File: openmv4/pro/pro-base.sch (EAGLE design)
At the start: 172 parts, among them J2 SAMTEC_FTSH-105-01-F-DVSAMTEC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, J6 RSP-122811-01, M1 9774030243R, M2 9774030243R, Q1 BSS138, Q2 AO3401, U1 W25Q256JVEIQ_TR, U10 STM32H743IIK6, U11 TEXAS_INSTRUMENTS_BQ24072TRGT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, U12 MICROCHIP_ATECC608A-SSHDA-BMI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, U14 IS42S32800, U2 EMIF06-MSD02N16, U3 ME6211C18M5G, U4 PAM2305AABADJ, U5 LSM6DS3TR-C, U6 MICROCHIP_USB3320C-EZK-TRMICR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, U7 LBEE5KL1DX-TEMP, U9 VL53L5CX, X2 USD-1040310811, X3 DF12-36-DS, X4 S2B-PH-K-S(LF)(SN), Y0 SITIME_SIT1533AI-H4-DCC-32.76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, Y1 DSC1001BI1-024.0000

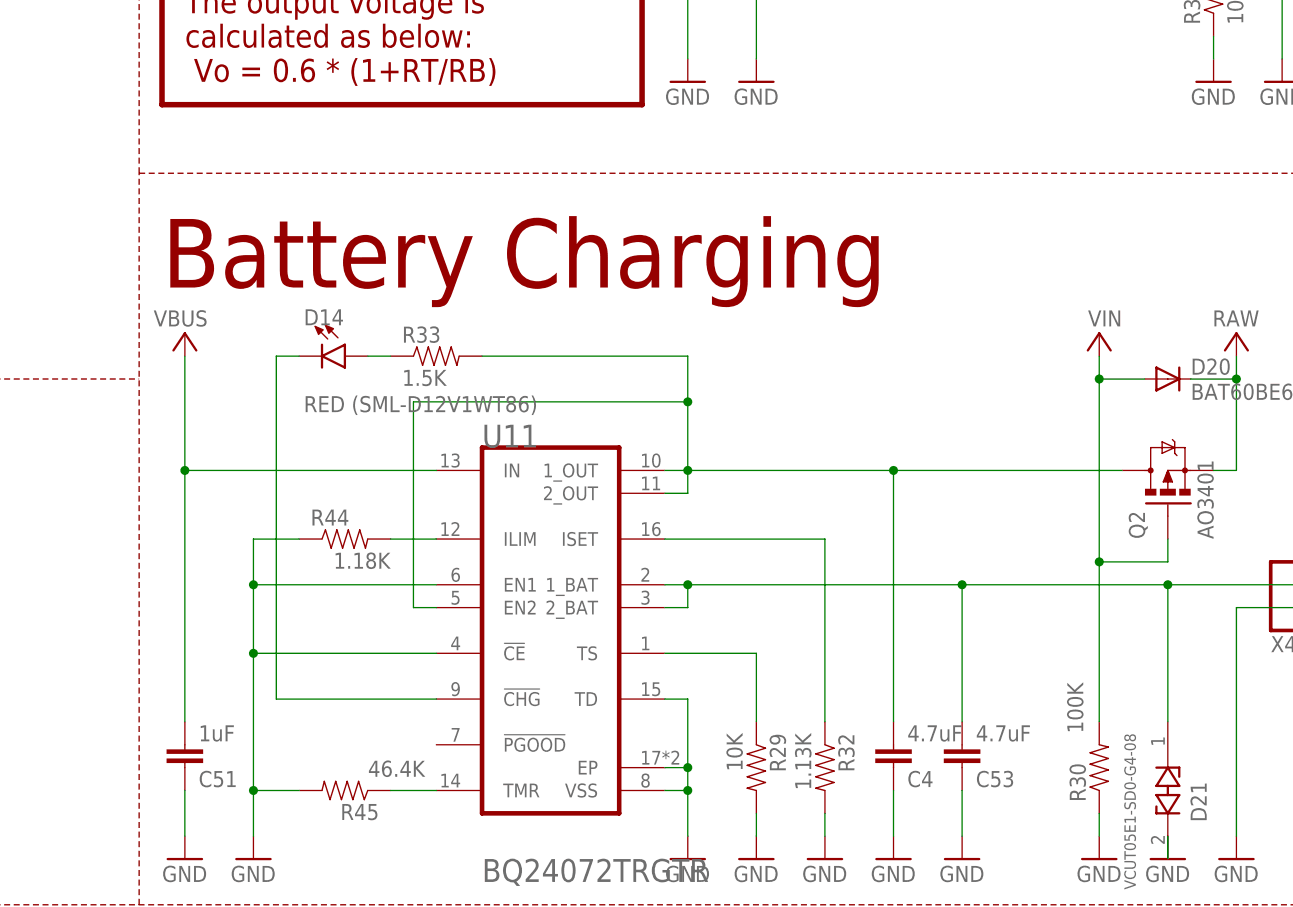
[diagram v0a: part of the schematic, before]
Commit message: Update pro schematics
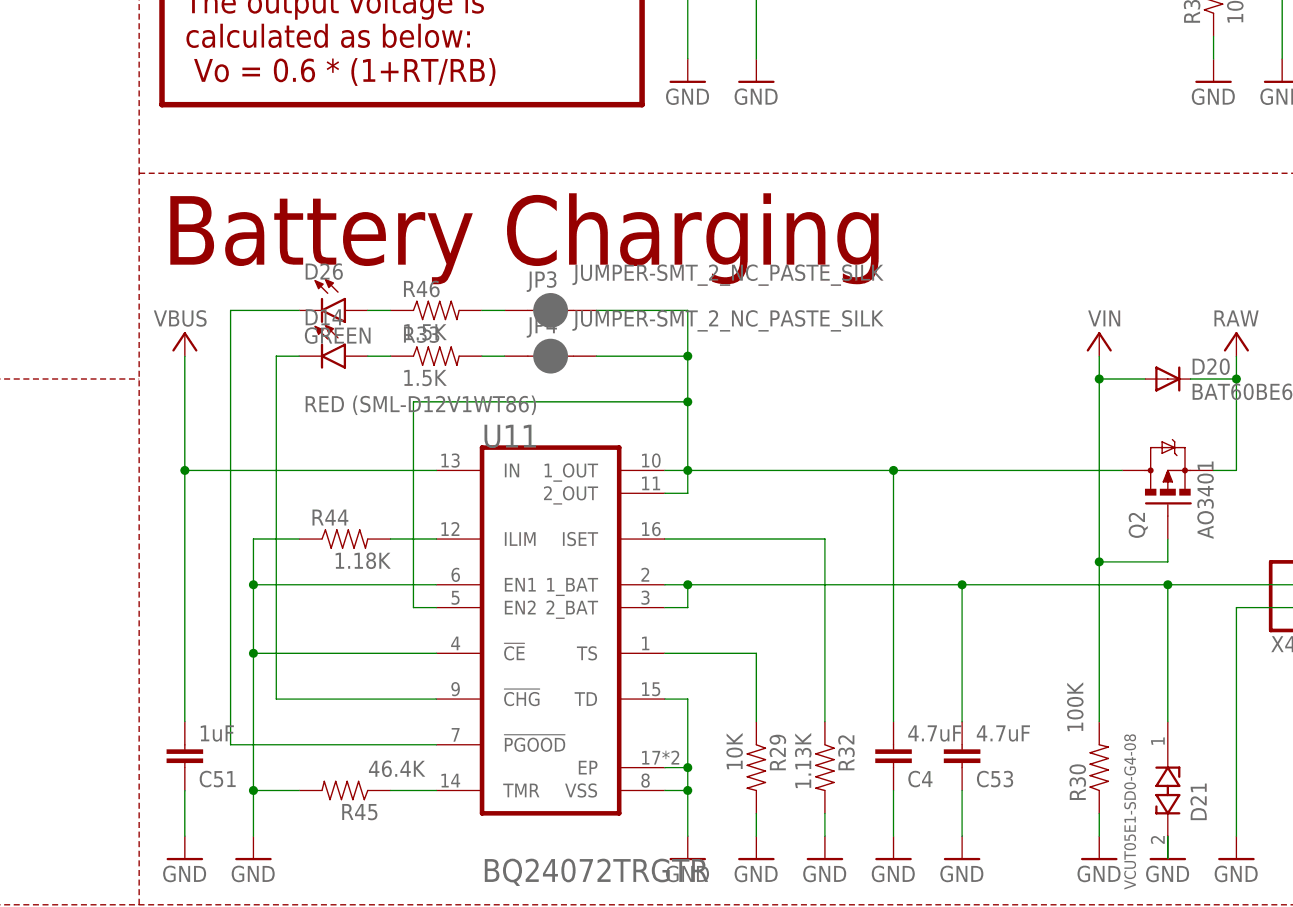
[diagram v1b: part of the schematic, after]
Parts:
- added D26: GREEN, SparkFun-LED:LED-GREEN0603
- added JP3, JP4: JUMPER-SMT_2_NC_PASTE_SILK, SparkFun-Jumpers:JUMPER-SMT_2_NC_PASTE_SILK
- added R46: 1.5K, sfe:RESISTOR0402-RES
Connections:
- new net N$1: D26.A, R46.1
- new net N$11: JP4.1, R33.2
- new net N$12: JP3.1, R46.2
- new net N$9: D26.C, U11.!PGOOD!
- net OUT: now also JP3.2, JP4.2; no longer R33.2
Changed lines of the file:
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@@
 <part name="R45" library="sfe" deviceset="RESISTOR" device="0402-RES" value="46.4K"/>
 <part name="J6" library="RSP-122811-01" deviceset="RSP-122811-01" device=""/>
+<part name="R46" library="sfe" deviceset="RESISTOR" device="0402-RES" value="1.5K"/>
+<part name="D26" library="SparkFun-LED" library_urn="urn:adsk.eagle:library:529" deviceset="LED-GREEN" device="0603" package3d_urn="urn:adsk.eagle:package:39354/1" value="GREEN"/>
+<part name="JP3" library="SparkFun-Jumpers" library_urn="urn:adsk.eagle:library:528" deviceset="JUMPER-SMT_2_NC_PASTE" device="_SILK" package3d_urn="urn:adsk.eagle:package:39282/1"/>
+<part name="JP4" library="SparkFun-Jumpers" library_urn="urn:adsk.eagle:library:528" deviceset="JUMPER-SMT_2_NC_PASTE" device="_SILK" package3d_urn="urn:adsk.eagle:package:39282/1"/>
 </parts>
 <sheets>
@@
 <text x="96.52" y="391.16" size="1.27" layer="150" font="vector" ratio="20">* Swapped to make
   layout easier</text>
-<text x="134.62" y="358.14" size="7.62" layer="94" font="vector" ratio="20">Battery Charging</text>
+<text x="134.62" y="360.68" size="7.62" layer="94" font="vector" ratio="20">Battery Charging</text>
 <wire x1="132.08" y1="370.84" x2="271.78" y2="370.84" width="0.1524" layer="94" style="longdash"/>
 <text x="134.62" y="419.1" size="7.62" layer="94" font="vector" ratio="20">Power</text>
@@
 <attribute name="VALUE" x="407.924" y="92.202" size="1.778" layer="96" rot="MR0"/>
 </instance>
+<instance part="R46" gate="G$1" x="165.1" y="355.6" smashed="yes">
+<attribute name="NAME" x="161.29" y="357.0986" size="1.778" layer="95"/>
+<attribute name="VALUE" x="161.29" y="352.298" size="1.778" layer="96"/>
+</instance>
+<instance part="D26" gate="G$1" x="154.94" y="355.6" smashed="yes" rot="R270">
+<attribute name="NAME" x="150.368" y="359.029" size="1.778" layer="95" font="vector"/>
+<attribute name="VALUE" x="150.368" y="353.695" size="1.778" layer="96" font="vector" align="top-left"/>
+</instance>
+<instance part="JP3" gate="G$1" x="177.8" y="355.6" smashed="yes">
+<attribute name="NAME" x="175.26" y="358.14" size="1.778" layer="95" font="vector"/>
+<attribute name="VALUE" x="180.34" y="360.68" size="1.778" layer="96" font="vector" align="top-left"/>
+</instance>
+<instance part="JP4" gate="G$1" x="177.8" y="350.52" smashed="yes">
+<attribute name="NAME" x="175.26" y="353.06" size="1.778" layer="95" font="vector"/>
+<attribute name="VALUE" x="180.34" y="355.6" size="1.778" layer="96" font="vector" align="top-left"/>
+</instance>
 </instances>
 <busses>
@@
 <wire x1="193.04" y1="337.82" x2="215.9" y2="337.82" width="0.1524" layer="91"/>
 <junction x="193.04" y="337.82"/>
-<wire x1="193.04" y1="350.52" x2="193.04" y2="345.44" width="0.1524" layer="91"/>
 <pinref part="C4" gate="G$1" pin="2"/>
 <wire x1="193.04" y1="345.44" x2="193.04" y2="337.82" width="0.1524" layer="91"/>
 <wire x1="215.9" y1="337.82" x2="241.3" y2="337.82" width="0.1524" layer="91"/>
 <junction x="215.9" y="337.82"/>
-<pinref part="R33" gate="G$1" pin="2"/>
-<wire x1="193.04" y1="350.52" x2="170.18" y2="350.52" width="0.1524" layer="91"/>
 <pinref part="U11" gate="G$0" pin="EN2"/>
 <wire x1="165.1" y1="322.58" x2="162.56" y2="322.58" width="0.1524" layer="91"/>
@@
 <wire x1="162.56" y1="345.44" x2="193.04" y2="345.44" width="0.1524" layer="91"/>
 <junction x="193.04" y="345.44"/>
+<wire x1="193.04" y1="355.6" x2="193.04" y2="350.52" width="0.1524" layer="91"/>
+<pinref part="JP3" gate="G$1" pin="2"/>
+<wire x1="193.04" y1="350.52" x2="193.04" y2="345.44" width="0.1524" layer="91"/>
+<wire x1="182.88" y1="355.6" x2="193.04" y2="355.6" width="0.1524" layer="91"/>
+<pinref part="JP4" gate="G$1" pin="2"/>
+<wire x1="182.88" y1="350.52" x2="193.04" y2="350.52" width="0.1524" layer="91"/>
+<junction x="193.04" y="350.52"/>
 </segment>
 </net>
@@
 </segment>
 </net>
+<net name="N$1" class="0">
+<segment>
+<pinref part="D26" gate="G$1" pin="A"/>
+<pinref part="R46" gate="G$1" pin="1"/>
+<wire x1="157.48" y1="355.6" x2="160.02" y2="355.6" width="0.1524" layer="91"/>
+</segment>
+</net>
+<net name="N$9" class="0">
+<segment>
+<pinref part="D26" gate="G$1" pin="C"/>
+<wire x1="149.86" y1="355.6" x2="142.24" y2="355.6" width="0.1524" layer="91"/>
+<wire x1="142.24" y1="355.6" x2="142.24" y2="307.34" width="0.1524" layer="91"/>
+<pinref part="U11" gate="G$0" pin="!PGOOD!"/>
+<wire x1="142.24" y1="307.34" x2="165.1" y2="307.34" width="0.1524" layer="91"/>
+</segment>
+</net>
+<net name="N$11" class="0">
+<segment>
+<pinref part="R33" gate="G$1" pin="2"/>
+<pinref part="JP4" gate="G$1" pin="1"/>
+<wire x1="170.18" y1="350.52" x2="172.72" y2="350.52" width="0.1524" layer="91"/>
+</segment>
+</net>
+<net name="N$12" class="0">
+<segment>
+<pinref part="R46" gate="G$1" pin="2"/>
+<pinref part="JP3" gate="G$1" pin="1"/>
+<wire x1="170.18" y1="355.6" x2="172.72" y2="355.6" width="0.1524" layer="91"/>
+</segment>
+</net>
